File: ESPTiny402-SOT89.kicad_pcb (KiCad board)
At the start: 2 copper layers, 26.4 x 23.9 mm, 21 parts, among them J1 Conn_01x10_Male, J2 Conn_01x10_Male, J3 Conn_01x04_Male, U1 ESP-01v090, U2 ATtiny402-SS, U3 MCP1700

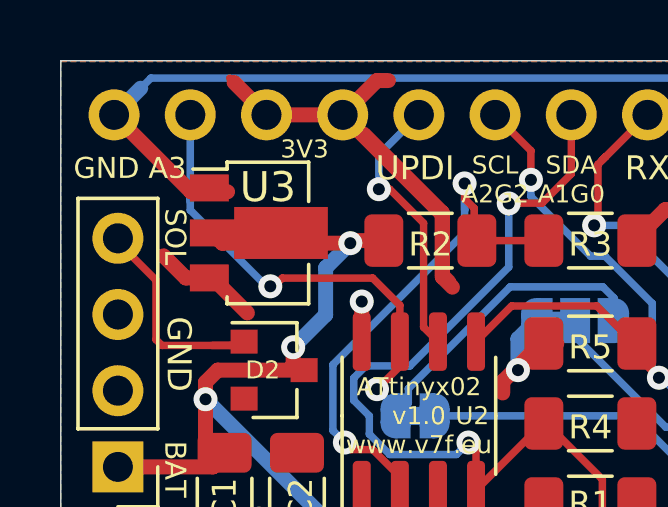
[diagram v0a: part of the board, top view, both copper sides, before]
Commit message: clean up
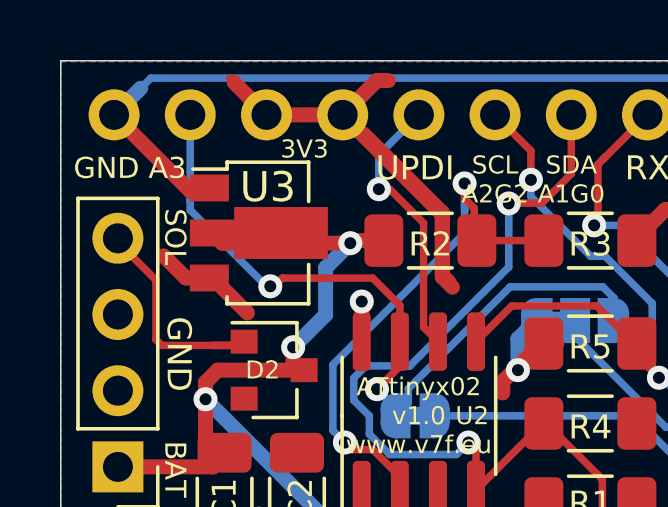
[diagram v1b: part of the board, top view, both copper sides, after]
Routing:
- net GND: track 103.8 -> 103.2 mm
